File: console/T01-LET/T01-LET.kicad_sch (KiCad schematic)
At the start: 16 parts, among them J1 RaspberryPi_ZERO_2_W, J10 Pasori_Cable, J11 MicroB_Cable, J2 MicroUSB_Port, J3 PP1, J4 PP3, J5 PP22, J6 PP23, J7 CP2102, J8 USB_C, M1 Motor_Servo, Q1 2SK4017

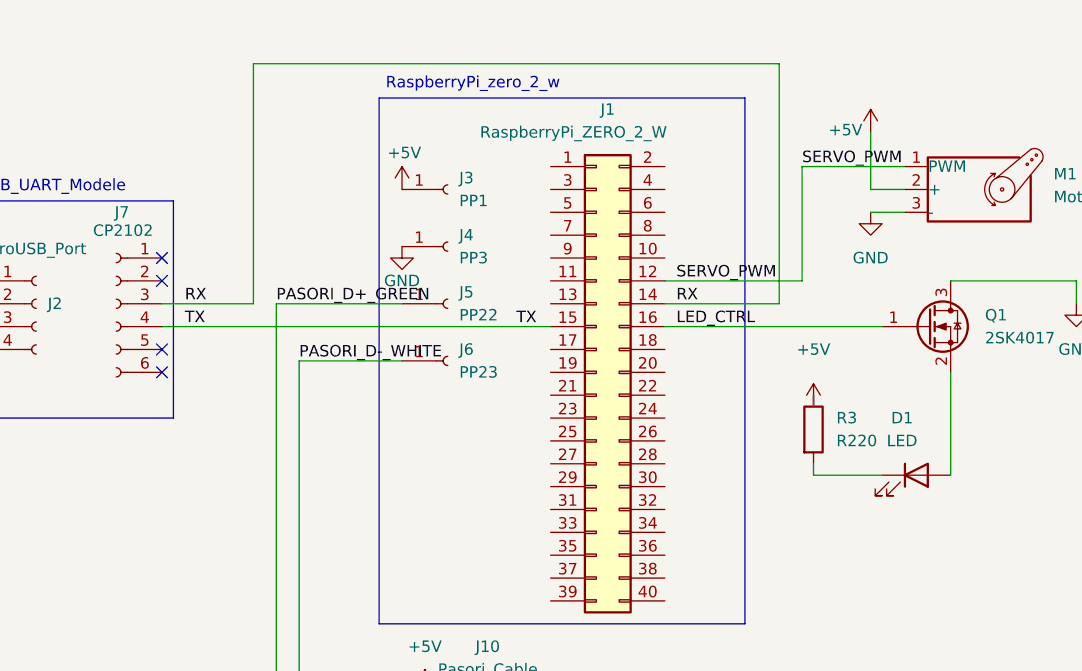
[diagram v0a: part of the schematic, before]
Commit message: v1.1.1: Release v1.1.1
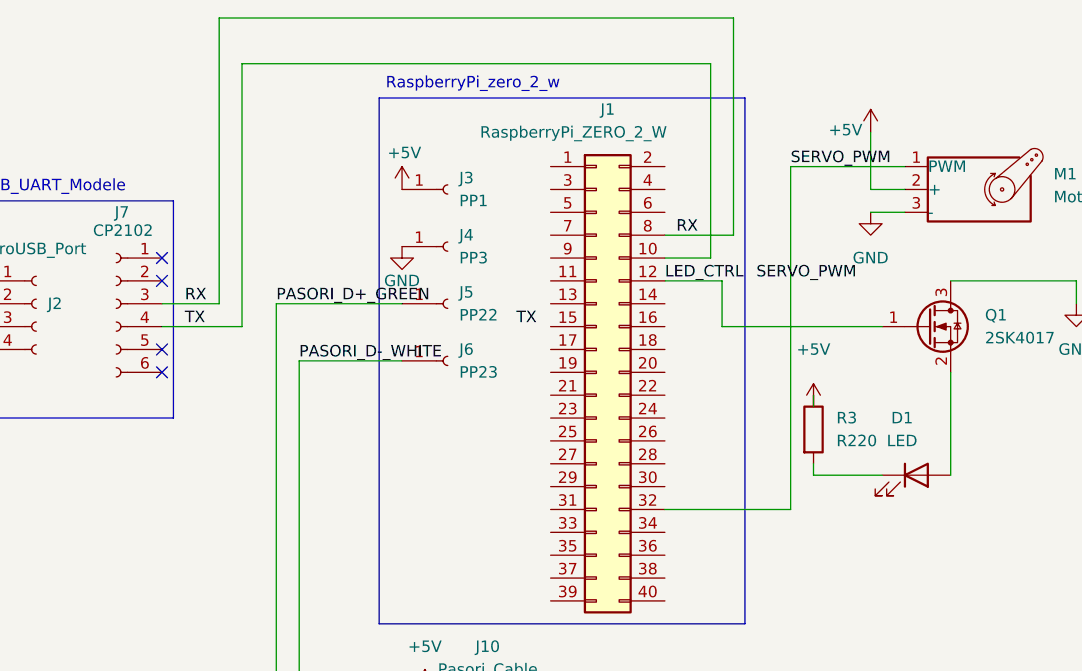
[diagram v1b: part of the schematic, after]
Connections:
- net LED_CTRL: now also J1.12 (Pin_12); no longer J1.16 (Pin_16)
- net RX: now also J1.8 (Pin_8); no longer J1.14 (Pin_14)
- net SERVO_PWM: now also J1.32 (Pin_32); no longer J1.12 (Pin_12)
- net TX: now also J1.10 (Pin_10); no longer J1.15 (Pin_15)
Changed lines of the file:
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@@
-	(wire
-		(pts
-			(xy 208.28 90.17) (xy 232.41 90.17)
-		)
-		(stroke
-			(width 0)
-			(type default)
-		)
-	)
 	(wire
 		(pts
@@
 	(wire
 		(pts
+			(xy 152.4 90.17) (xy 161.29 90.17)
+		)
+		(stroke
+			(width 0)
+			(type default)
+		)
+	)
+	(wire
+		(pts
 			(xy 189.23 138.43) (xy 195.58 138.43)
 		)
@@
 	(wire
 		(pts
-			(xy 223.52 72.39) (xy 234.95 72.39)
+			(xy 222.25 72.39) (xy 234.95 72.39)
+		)
+		(stroke
+			(width 0)
+			(type default)
+		)
+	)
+	(wire
+		(pts
+			(xy 214.63 90.17) (xy 214.63 85.09)
 		)
 		(stroke
@@
 	(wire
 		(pts
+			(xy 161.29 60.96) (xy 213.36 60.96)
+		)
+		(stroke
+			(width 0)
+			(type default)
+		)
+	)
+	(wire
+		(pts
 			(xy 231.14 68.58) (xy 231.14 74.93)
 		)
@@
 	(wire
 		(pts
-			(xy 162.56 60.96) (xy 220.98 60.96)
+			(xy 222.25 110.49) (xy 208.28 110.49)
+		)
+		(stroke
+			(width 0)
+			(type default)
+		)
+	)
+	(wire
+		(pts
+			(xy 232.41 90.17) (xy 214.63 90.17)
+		)
+		(stroke
+			(width 0)
+			(type default)
+		)
+	)
+	(wire
+		(pts
+			(xy 158.75 55.88) (xy 215.9 55.88)
 		)
 		(stroke
@@
 	(wire
 		(pts
-			(xy 152.4 90.17) (xy 195.58 90.17)
-		)
-		(stroke
-			(width 0)
-			(type default)
-		)
-	)
-	(wire
-		(pts
 			(xy 189.23 135.89) (xy 195.58 135.89)
 		)
@@
 	(wire
 		(pts
-			(xy 162.56 87.63) (xy 152.4 87.63)
+			(xy 158.75 87.63) (xy 152.4 87.63)
 		)
 		(stroke
@@
 	(wire
 		(pts
-			(xy 220.98 60.96) (xy 220.98 87.63)
+			(xy 215.9 55.88) (xy 215.9 80.01)
+		)
+		(stroke
+			(width 0)
+			(type default)
+		)
+	)
+	(wire
+		(pts
+			(xy 208.28 82.55) (xy 213.36 82.55)
 		)
 		(stroke
@@
 	(wire
 		(pts
-			(xy 223.52 85.09) (xy 208.28 85.09)
-		)
-		(stroke
-			(width 0)
-			(type default)
-		)
-	)
-	(wire
-		(pts
 			(xy 81.28 86.36) (xy 87.63 86.36)
 		)
@@
 	(wire
 		(pts
-			(xy 223.52 72.39) (xy 223.52 85.09)
+			(xy 222.25 72.39) (xy 222.25 110.49)
 		)
 		(stroke
@@
 	(wire
 		(pts
+			(xy 161.29 90.17) (xy 161.29 60.96)
+		)
+		(stroke
+			(width 0)
+			(type default)
+		)
+	)
+	(wire
+		(pts
 			(xy 254 85.09) (xy 254 87.63)
 		)
@@
 	(wire
 		(pts
-			(xy 162.56 60.96) (xy 162.56 87.63)
-		)
-		(stroke
-			(width 0)
-			(type default)
-		)
-	)
-	(wire
-		(pts
-			(xy 220.98 87.63) (xy 208.28 87.63)
+			(xy 158.75 55.88) (xy 158.75 87.63)
+		)
+		(stroke
+			(width 0)
+			(type default)
+		)
+	)
+	(wire
+		(pts
+			(xy 215.9 80.01) (xy 208.28 80.01)
 		)
 		(stroke
@@
 	(wire
 		(pts
+			(xy 213.36 60.96) (xy 213.36 82.55)
+		)
+		(stroke
+			(width 0)
+			(type default)
+		)
+	)
+	(wire
+		(pts
 			(xy 50.8 91.44) (xy 76.2 91.44)
+		)
+		(stroke
+			(width 0)
+			(type default)
+		)
+	)
+	(wire
+		(pts
+			(xy 214.63 85.09) (xy 208.28 85.09)
 		)
 		(stroke
@@
 	)
 	(label "SERVO_PWM"
-		(at 223.52 72.39 0)
+		(at 222.25 72.39 0)
 		(effects
 			(font
@@
 	)
 	(label "RX"
-		(at 209.55 87.63 0)
+		(at 209.55 80.01 0)
 		(effects
 			(font
@@
 	)
 	(label "SERVO_PWM"
-		(at 209.55 85.09 0)
+		(at 218.44 85.09 0)
 		(effects
 			(font
@@
 	)
 	(label "LED_CTRL"
-		(at 209.55 90.17 0)
-		(effects
-			(font
+		(at 208.28 85.09 0)
+		(effects
+			(font
